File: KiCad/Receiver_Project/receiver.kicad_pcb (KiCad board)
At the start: 2 copper layers, 139.7 x 44.5 mm, 52 parts, among them J1 RB1-125BAG1A, Q1 PN2369A, Q2 2N3904, Q3 2N3904, Q4 2N3904, Q5 2N3904, Q6 2N3904, Q7 PN2369A, Q8 2N3904, Q9 PN2369A, U1 MC7805CTG, U2 LM7171, U3 LM7171, U4 Physical_Mount, U5 Physical_Mount

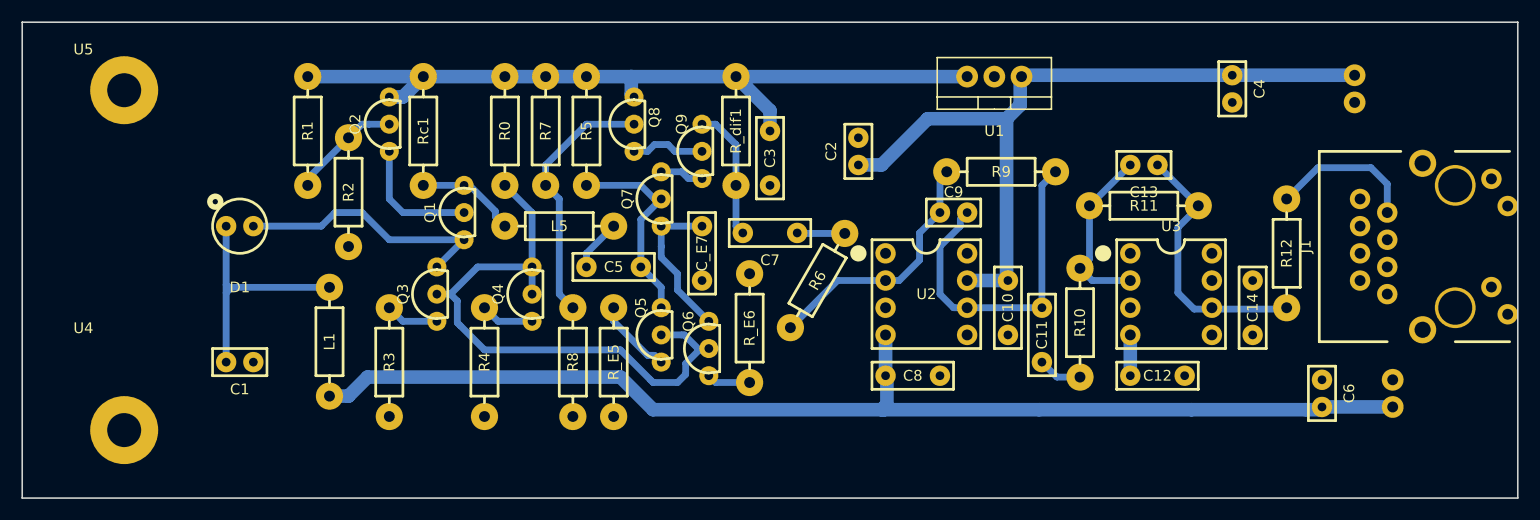
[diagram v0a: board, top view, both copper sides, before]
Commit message: receiver milled
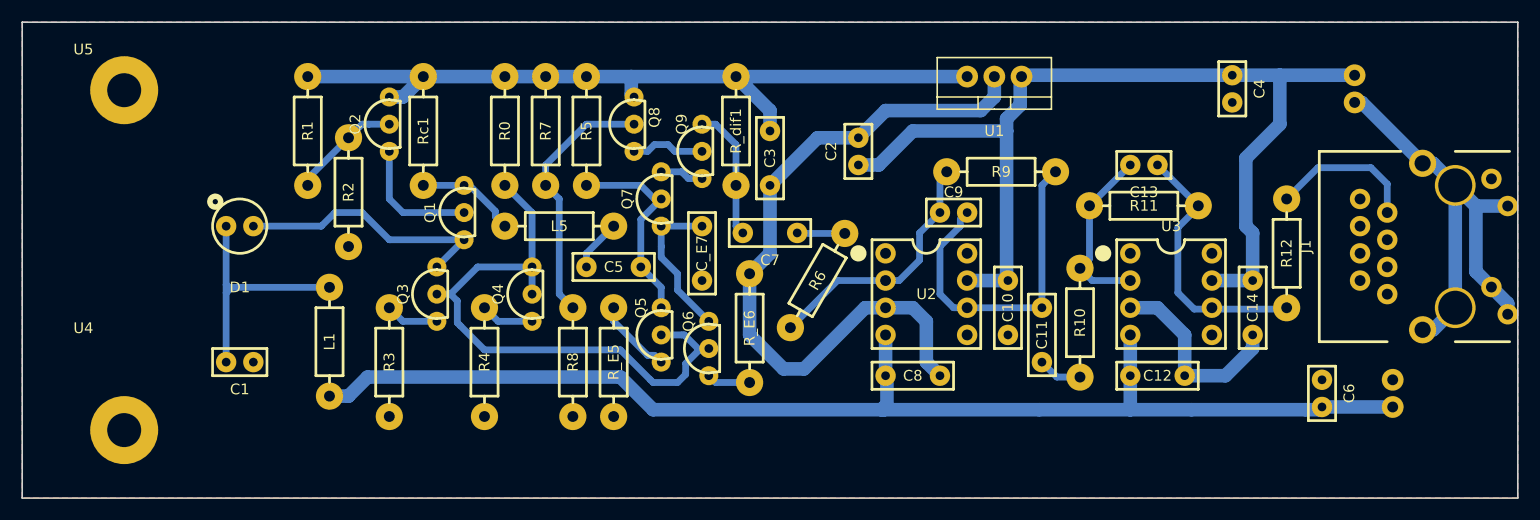
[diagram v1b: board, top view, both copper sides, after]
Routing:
- net GND: track 0.00 -> 133.7 mm
- net +9V: track 70.3 -> 94.4 mm
- net -9V: track 112.8 -> 115.9 mm
- added copper zone on B.Cu, net GND
- added copper zone on F.Cu, net GND

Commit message: added simulation labels to receiver schematic
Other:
- board text added: "Receiver PCB"
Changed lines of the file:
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@@
     (area 43.994714 68.905 208.330715 130.250001)
     (thickness 1.6)
-    (drawings 6)
+    (drawings 7)
     (tracks 221)
     (zones 0)
@@
       (net 2 GND))
   )
+  (gr_text "Receiver PCB" (at 215.9 174.625) (layer Dwgs.User)
+    (effects (font (size 5.3594 5.3594) (thickness 1.016)))
+  )
   (dimension 44.45 (width 0.3) (layer Dwgs.User)
